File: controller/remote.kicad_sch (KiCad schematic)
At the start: 11 parts, among them J1 Conn_01x03, U6 MC130VX

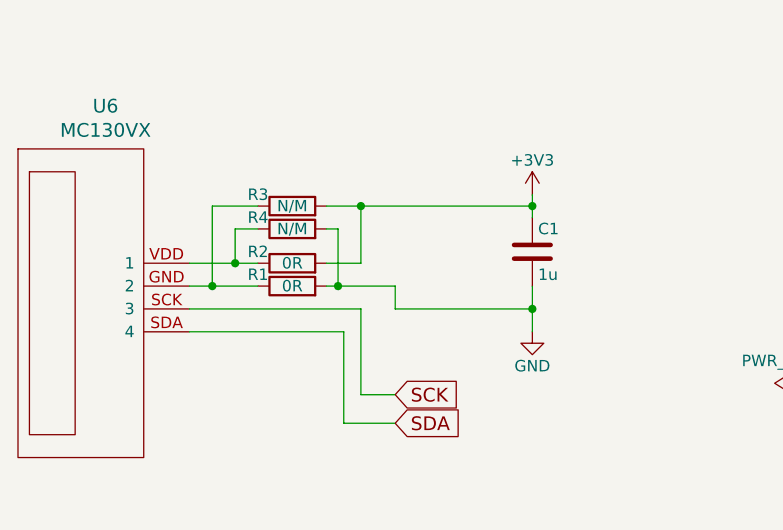
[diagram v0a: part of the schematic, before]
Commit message: Work on routing.
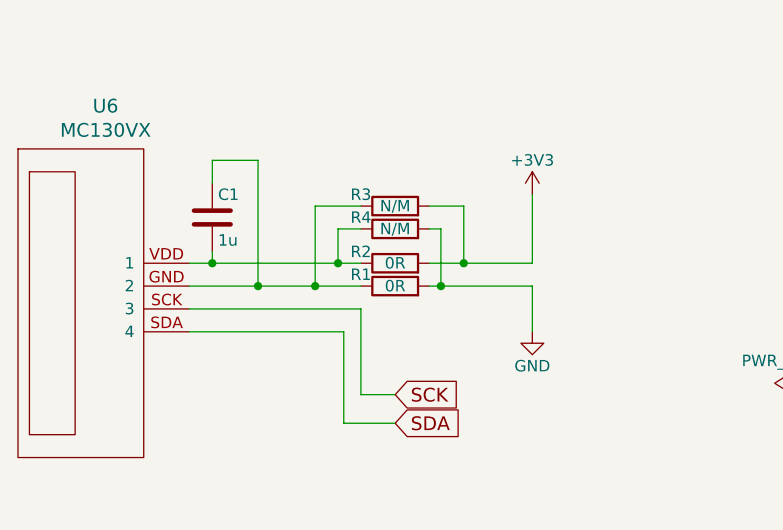
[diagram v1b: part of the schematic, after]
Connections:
- net +3V3: no longer C1.1
- net GND: no longer C1.2
- net at R1.1, R3.1, U6.GND (2): now also C1.1
- net at R2.1, R4.1, U6.VDD (1): now also C1.2
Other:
- moved on the sheet: C1, R1, R2, R3, R4
